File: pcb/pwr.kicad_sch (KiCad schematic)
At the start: 3 parts, among them J10 Barrel_Jack_Switch, J11 Screw_Terminal_01x02, Q9 Q_PMOS_GDS

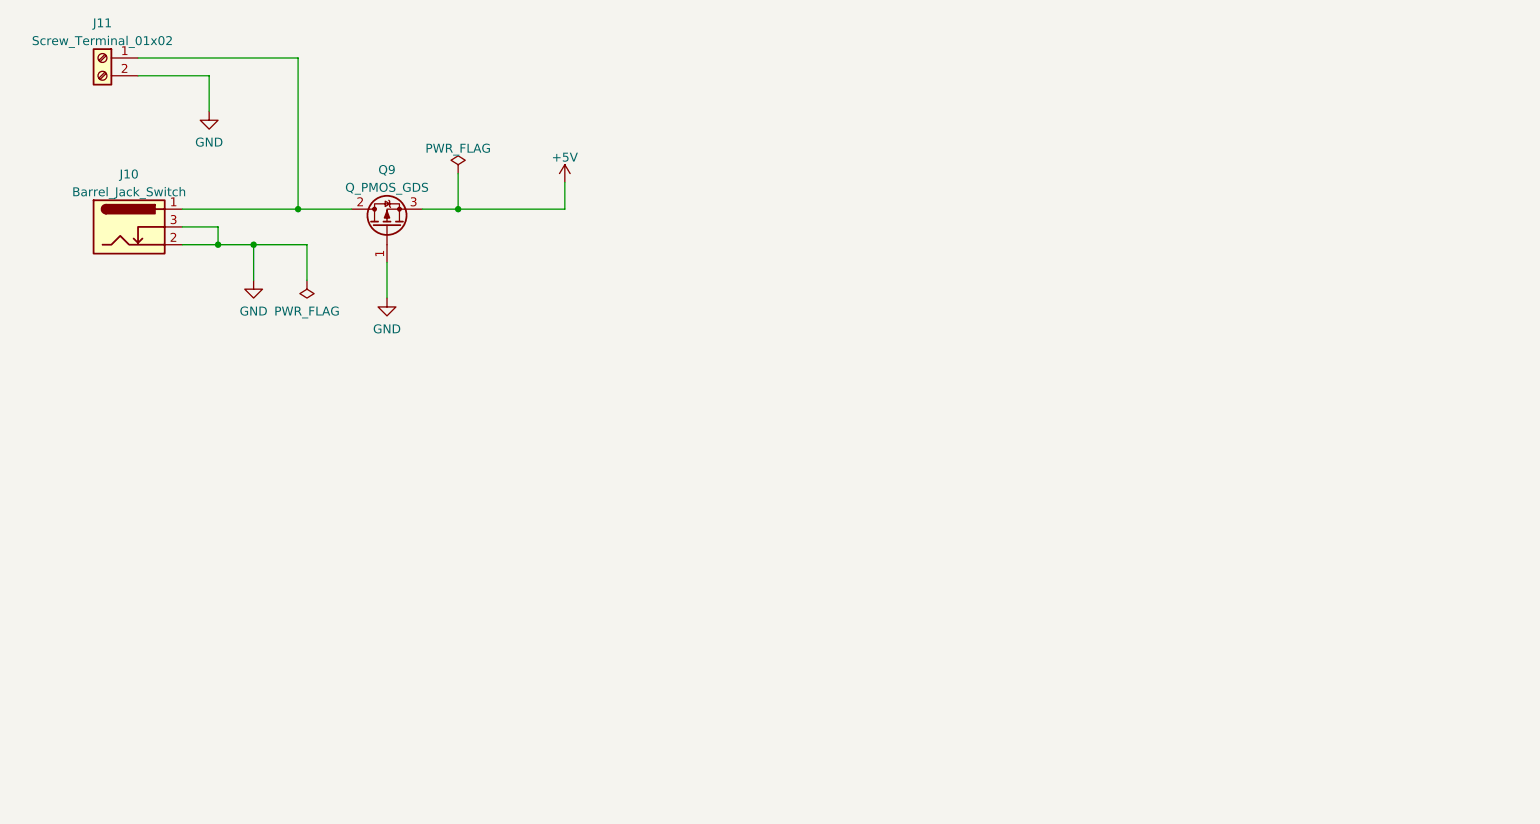
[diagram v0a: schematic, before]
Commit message: new layout with usb
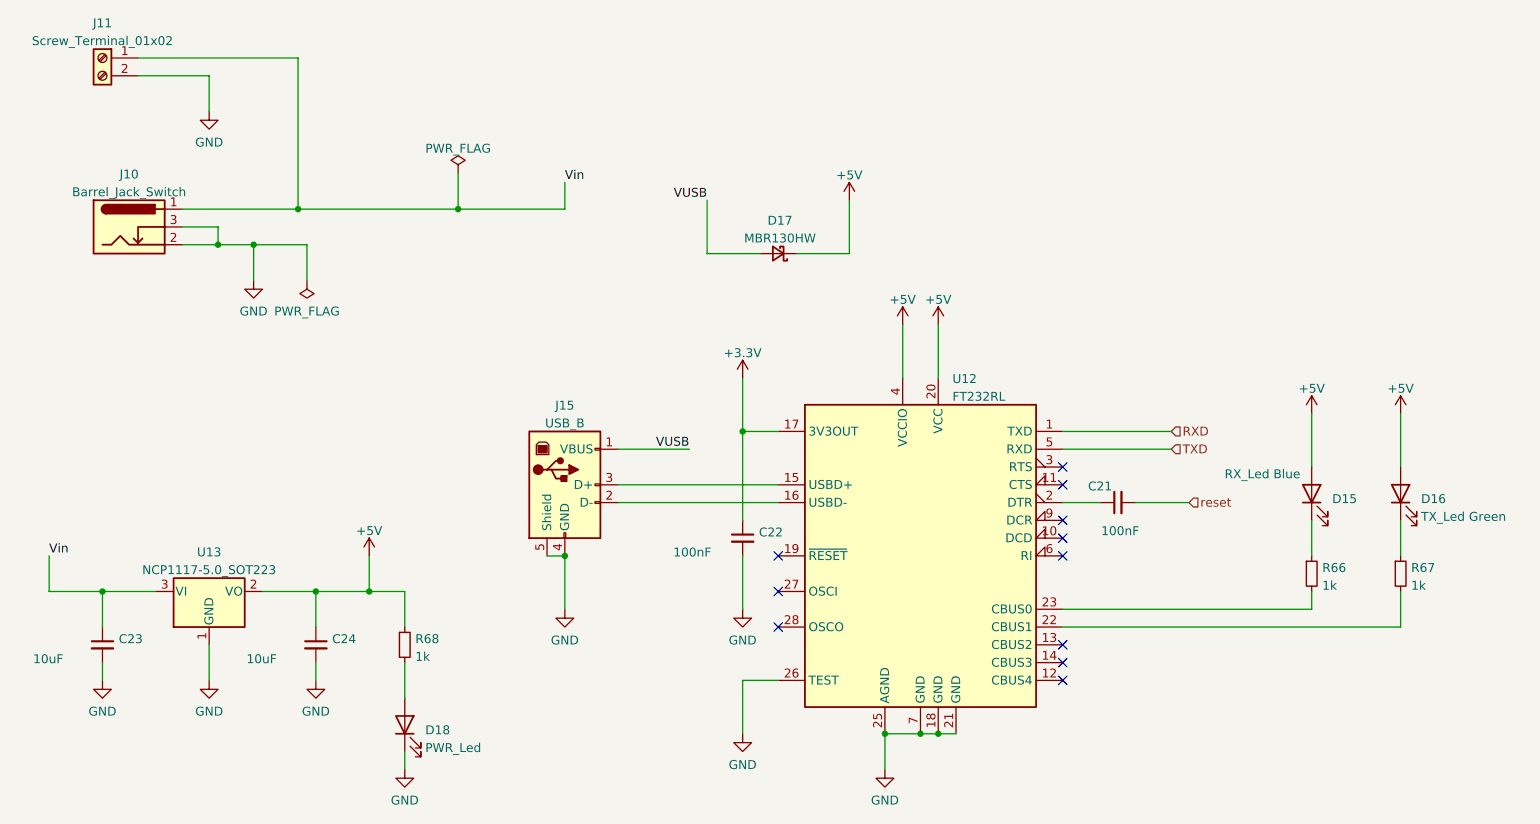
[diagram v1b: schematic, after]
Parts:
- removed Q9: Q_PMOS_GDS, Package_TO_SOT_THT:TO-220-3_Horizontal_TabDown, symbol Device:Q_PMOS_GDS
- added C21, C22: 100nF, Capacitor_SMD:C_0805_2012Metric_Pad1.18x1.45mm_HandSolder, symbol Device:C_Small
- added C23, C24: 10uF, Capacitor_SMD:C_0805_2012Metric_Pad1.18x1.45mm_HandSolder, symbol Device:C_Small
- added D15: RX_Led Blue, LED_SMD:LED_0805_2012Metric_Pad1.15x1.40mm_HandSolder, symbol Device:LED
- added D16: TX_Led Green, LED_SMD:LED_0805_2012Metric_Pad1.15x1.40mm_HandSolder, symbol Device:LED
- added D17: MBR130HW, Diode_SMD:D_SOD-123, symbol Device:D_Schottky_Small
- added D18: PWR_Led, LED_SMD:LED_0805_2012Metric_Pad1.15x1.40mm_HandSolder, symbol Device:LED
- added J15: USB_B, Connector_USB:USB_B_OST_USB-B1HSxx_Horizontal, symbol Connector:USB_B
- added R66, R67, R68: 1k, Resistor_SMD:R_0805_2012Metric_Pad1.20x1.40mm_HandSolder, symbol Device:R_Small
- added U12: FT232RL, Package_SO:SSOP-28_5.3x10.2mm_P0.65mm, symbol Interface_USB:FT232RL
- added U13: NCP1117-5.0_SOT223, Package_TO_SOT_SMD:SOT-223-3_TabPin2, symbol Regulator_Linear:NCP1117-5.0_SOT223
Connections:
- net +5V: now also C24.1, D15.2 (A), D16.2 (A), D17.1 (K), R68.1, U12.20 (VCC), U12.4 (VCCIO), U13.2 (VO)
- net GND: now also C22.2, C23.2, C24.2, D18.1 (K), J15.4 (GND), J15.5 (Shield), U12.18 (GND), U12.21 (GND), U12.25 (AGND), U12.26 (TEST), U12.7 (GND), U13.1 (GND)
- net Vin: now reaches J10.1, J11.1 (Pin_1)
- net Vin: now also C23.1, U13.3 (VI)
- new net: D15.1 (K), R66.1
- new net: R66.2, U12.23 (CBUS0)
- new net: J15.3 (D+), U12.15 (USBD+)
- new net: J15.2 (D-), U12.16 (USBD-)
- new net: C21.1, U12.2 (DTR)
- new net: R67.2, U12.22 (CBUS1)
- new net: D16.1 (K), R67.1
- new net: D18.2 (A), R68.2
- new net +3.3V: C22.1, U12.17 (3V3OUT)
- new net RXD: U12.1 (TXD)
- new net TXD: U12.5 (RXD)
- new net VUSB: D17.2 (A), J15.1 (VBUS)
- new net reset: C21.2
- no-connect marks 0 -> 11
